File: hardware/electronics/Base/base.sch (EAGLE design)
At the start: 45 parts, among them IC1 7805T, IC2 74LS595D, IC3 74LS595D, IC4 74LS595D

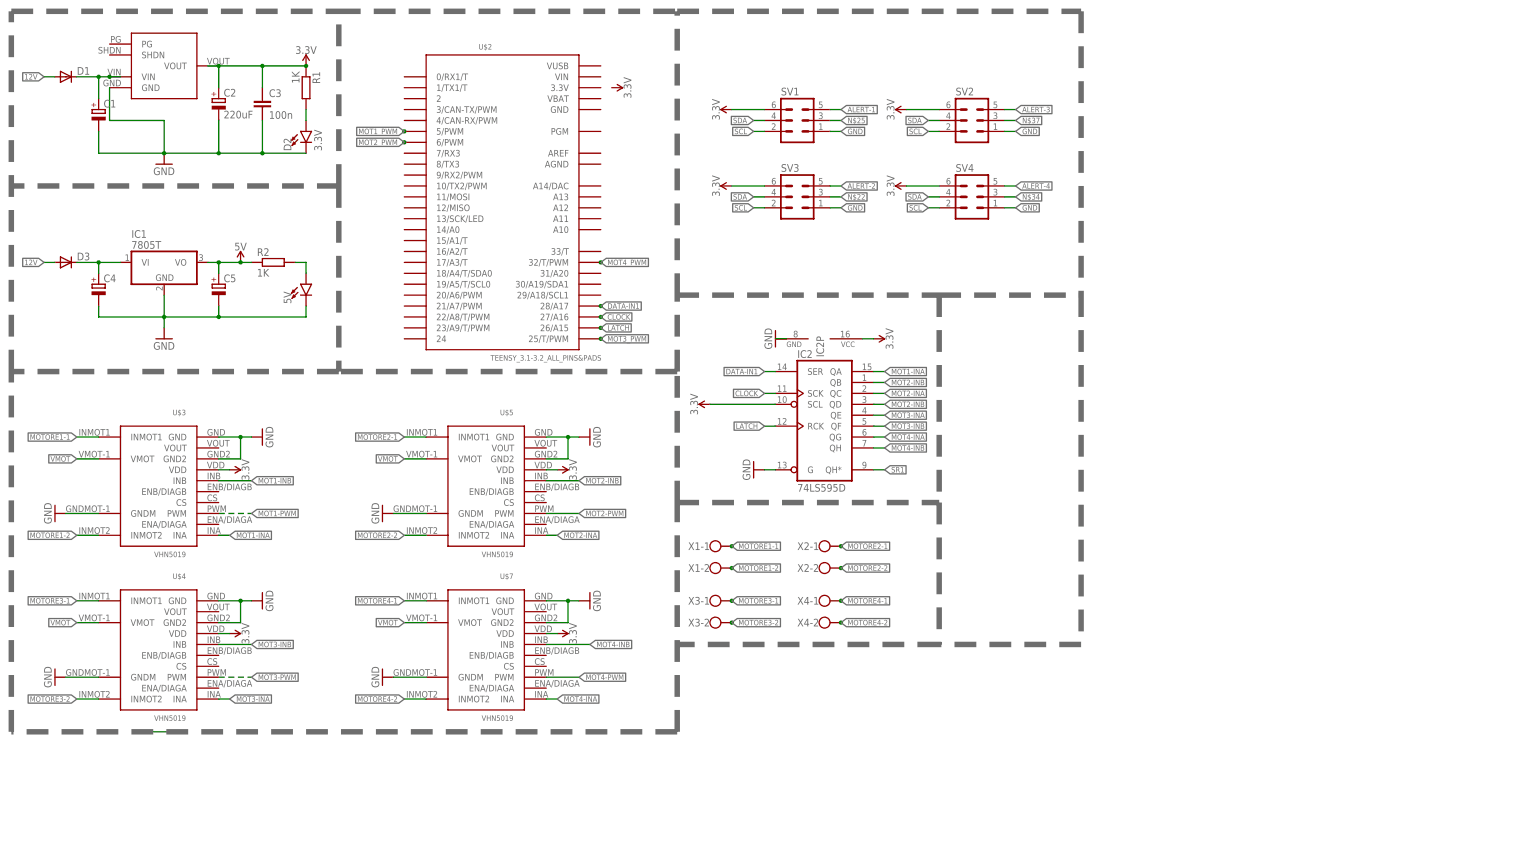
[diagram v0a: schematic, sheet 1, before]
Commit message: Base
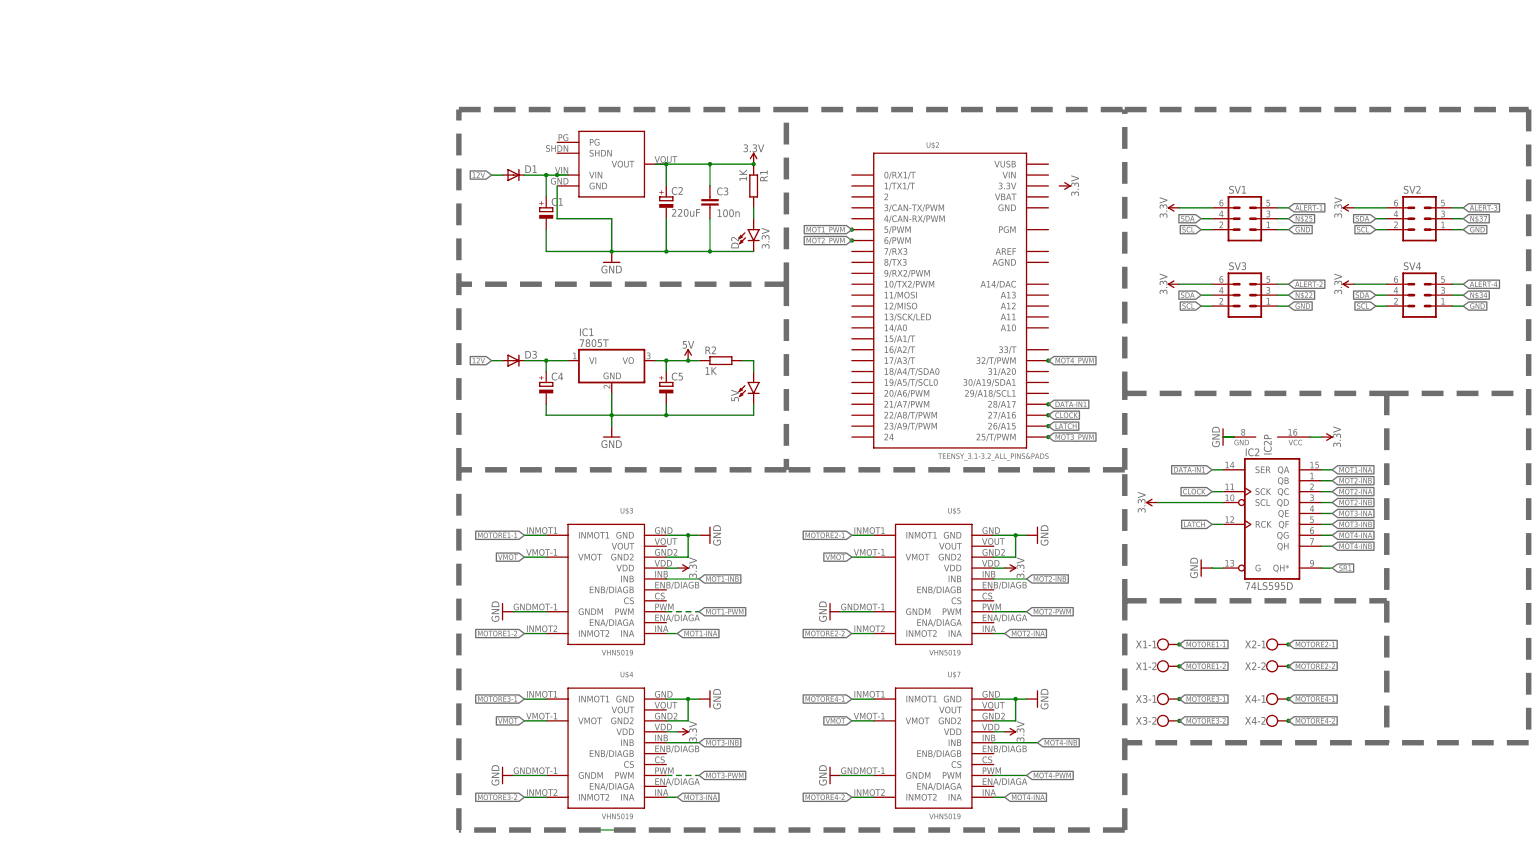
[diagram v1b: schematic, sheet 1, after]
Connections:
- net DIODO-1 renamed LED-1
- net DIODO-2 renamed LED-2
- net DIODO-3 renamed LED-3
- net DIODO-4 renamed LED-4
- net DIODO-5 renamed LED-5
- net DIODO-6 renamed LED-6
- net DIODO-7 renamed LED-7
- net DIODO-8 renamed LED-8
- removed net N$10: IC4A.SER
- new net SR2: IC3A.QH*, IC4A.SER
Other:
- note added: "Led segnalazione"
- note added: "Shift register"
- note added: "Shift register led"
- moved on the sheet: 5V, C1, C2, C3, C4, C5, D1, D10, D11, D12, D2, D3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
